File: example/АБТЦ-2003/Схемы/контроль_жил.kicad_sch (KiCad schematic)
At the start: 33 parts

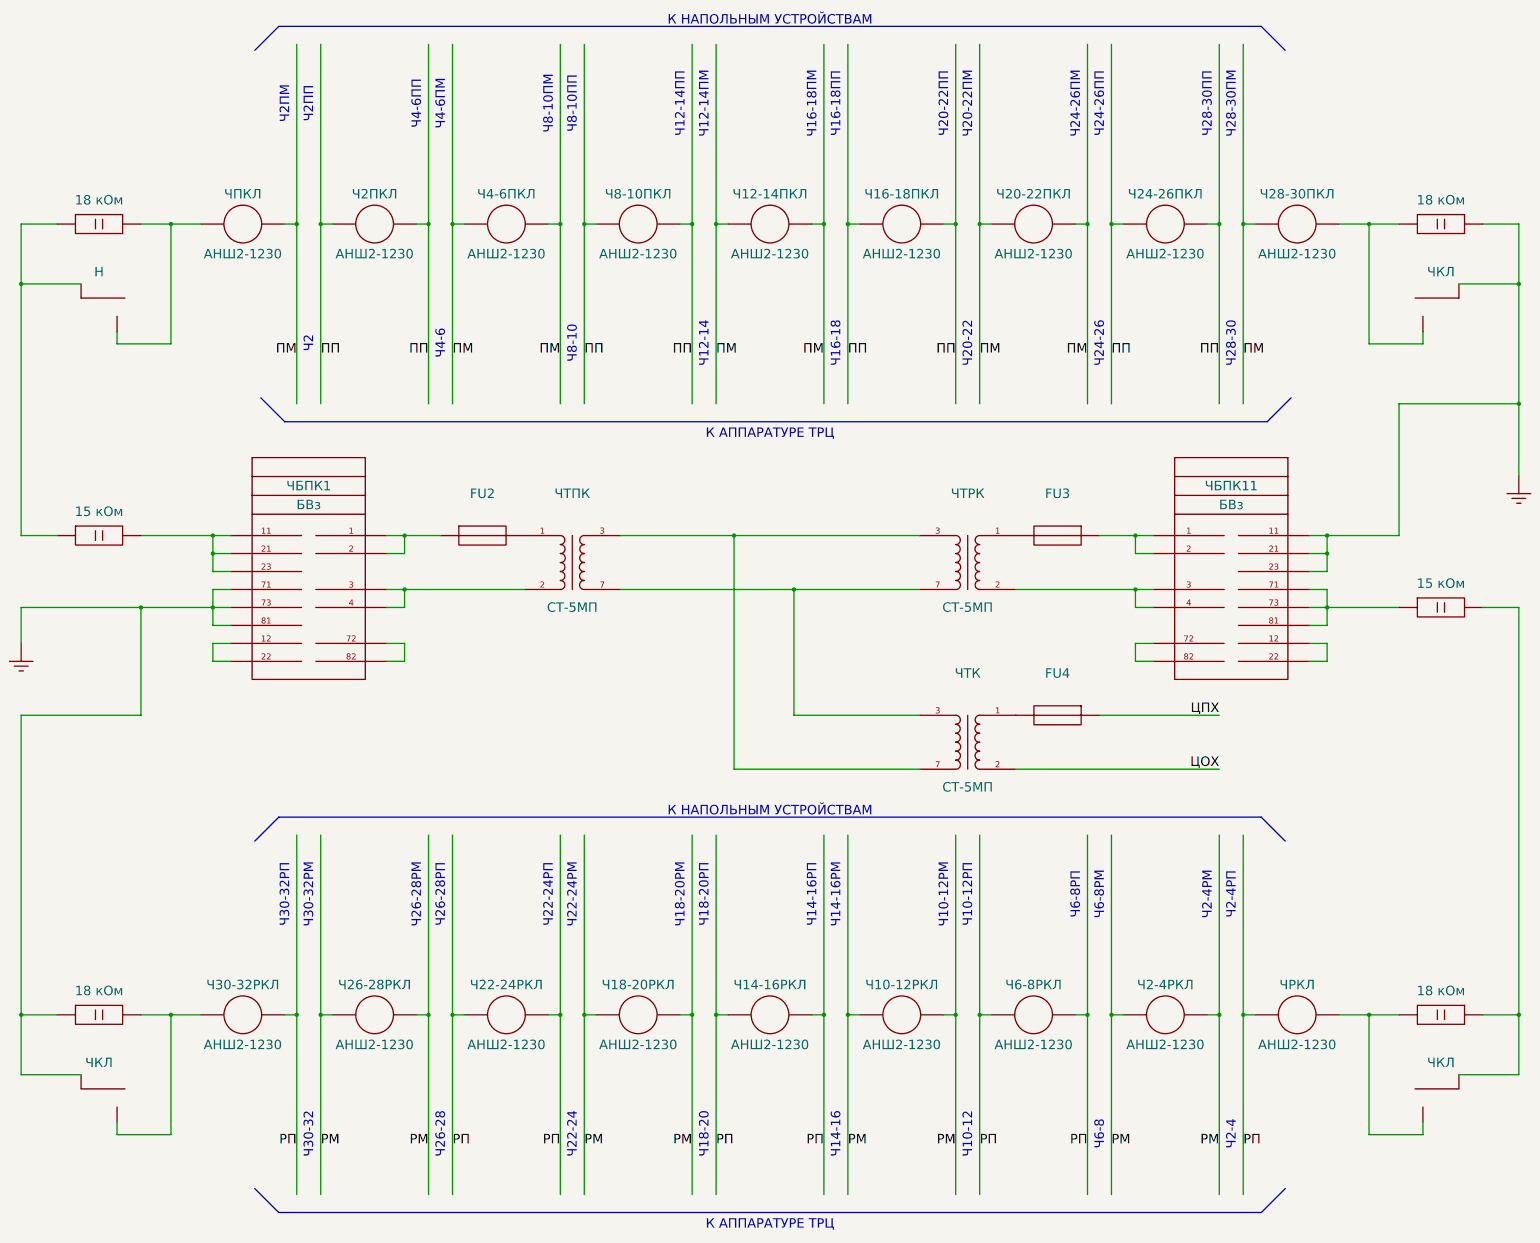
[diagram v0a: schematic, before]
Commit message: Шаблон АБТЦ обновлен
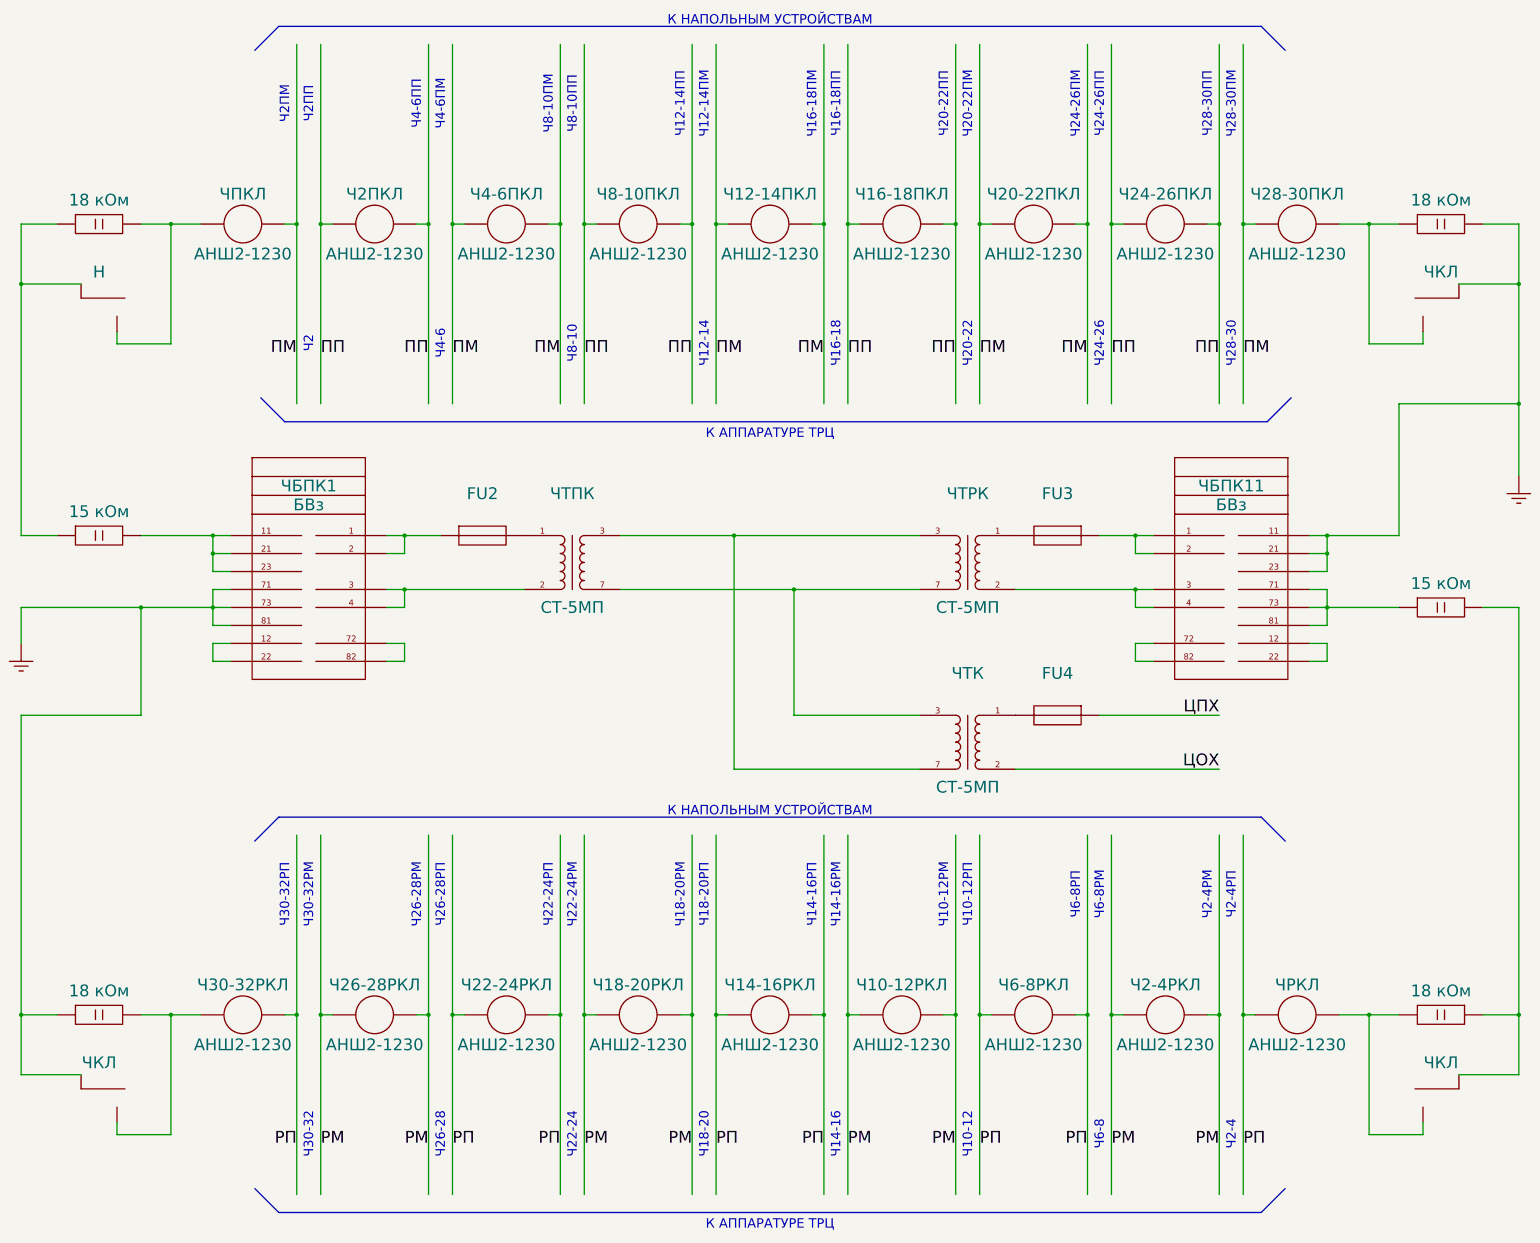
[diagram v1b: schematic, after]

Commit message: Обновление примера
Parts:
- Н1, Н11: symbol SCB_Relay:Контакт_нейтрального_якоря_НЗ -> SCB_Legacy:Контакт_нейтрального_якоря_НЗ_бн
